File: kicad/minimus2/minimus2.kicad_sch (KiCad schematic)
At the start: 35 parts, among them J1 PROG_SER, J4 Conn_01x01, J5 Conn_01x01, J6 Conn_01x01, J7 Conn_01x01, Q1 DMN3051L, Q2 AO3401A, Q3 SFH309, Q4 SFH309, Q5 SFH309, Q6 SFH309, Q7 DMN3051L, Q8 DMN3051L, Q9 DMN3051L, SW1 USER_A, SW2 RESET, U1 DRV8835, U2 LSM6DSRTR, U4 AS5047D, U5 AS5047D, U6 STM32U575CITx

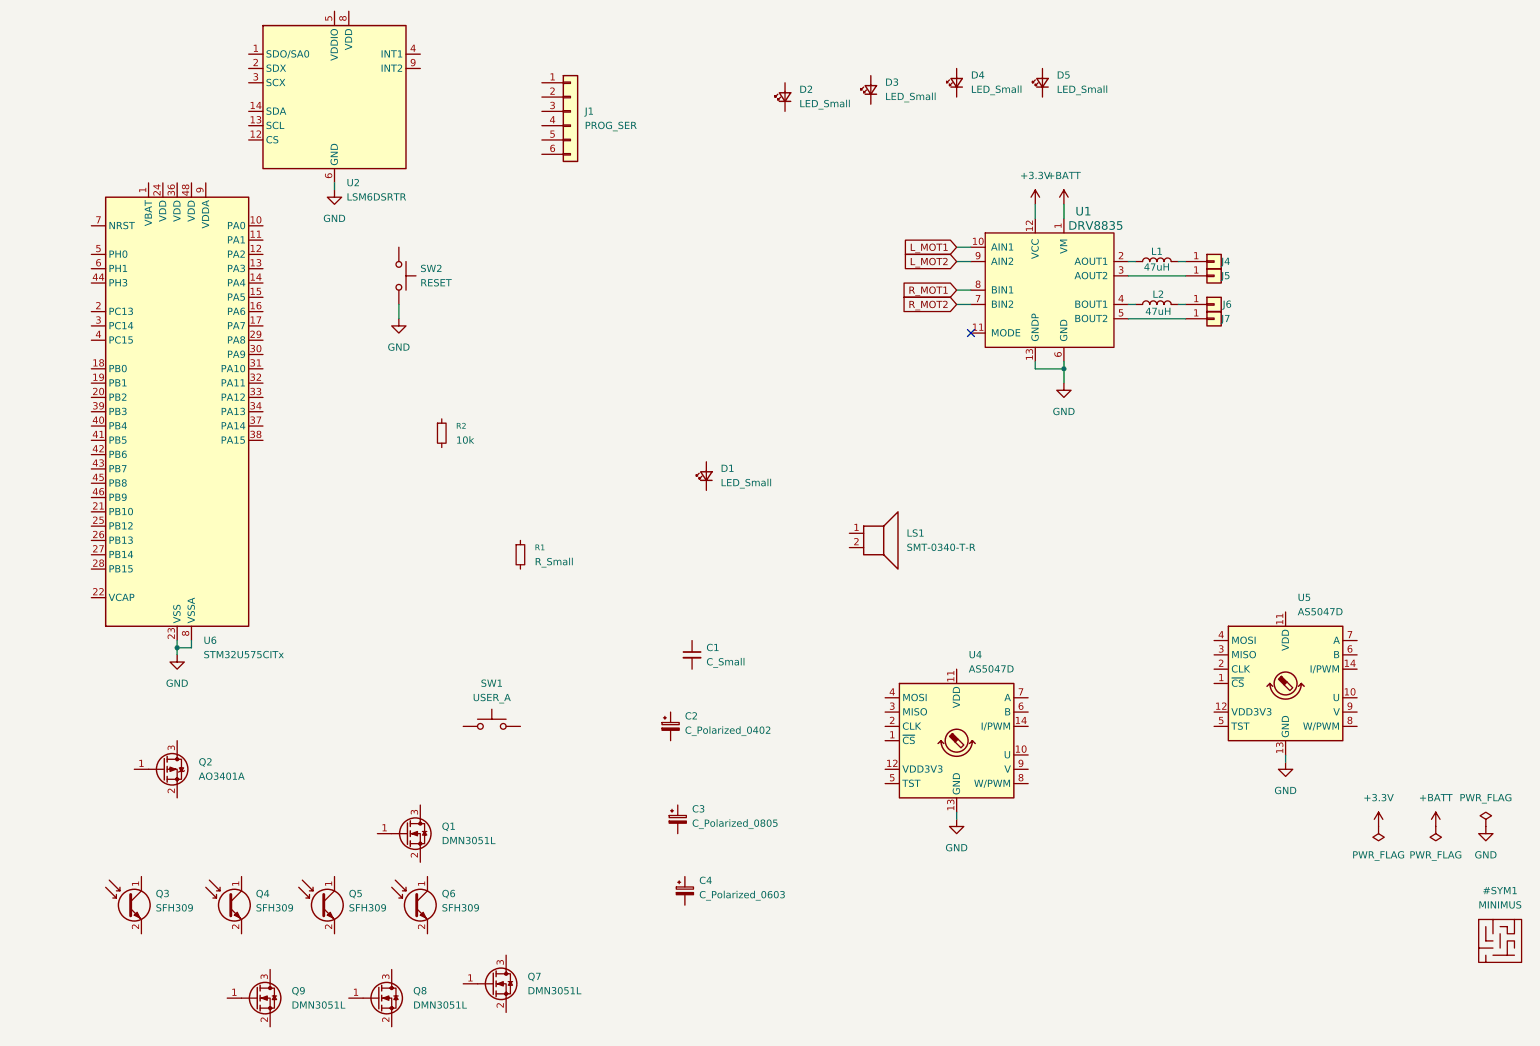
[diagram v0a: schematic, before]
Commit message: Rough place most parts
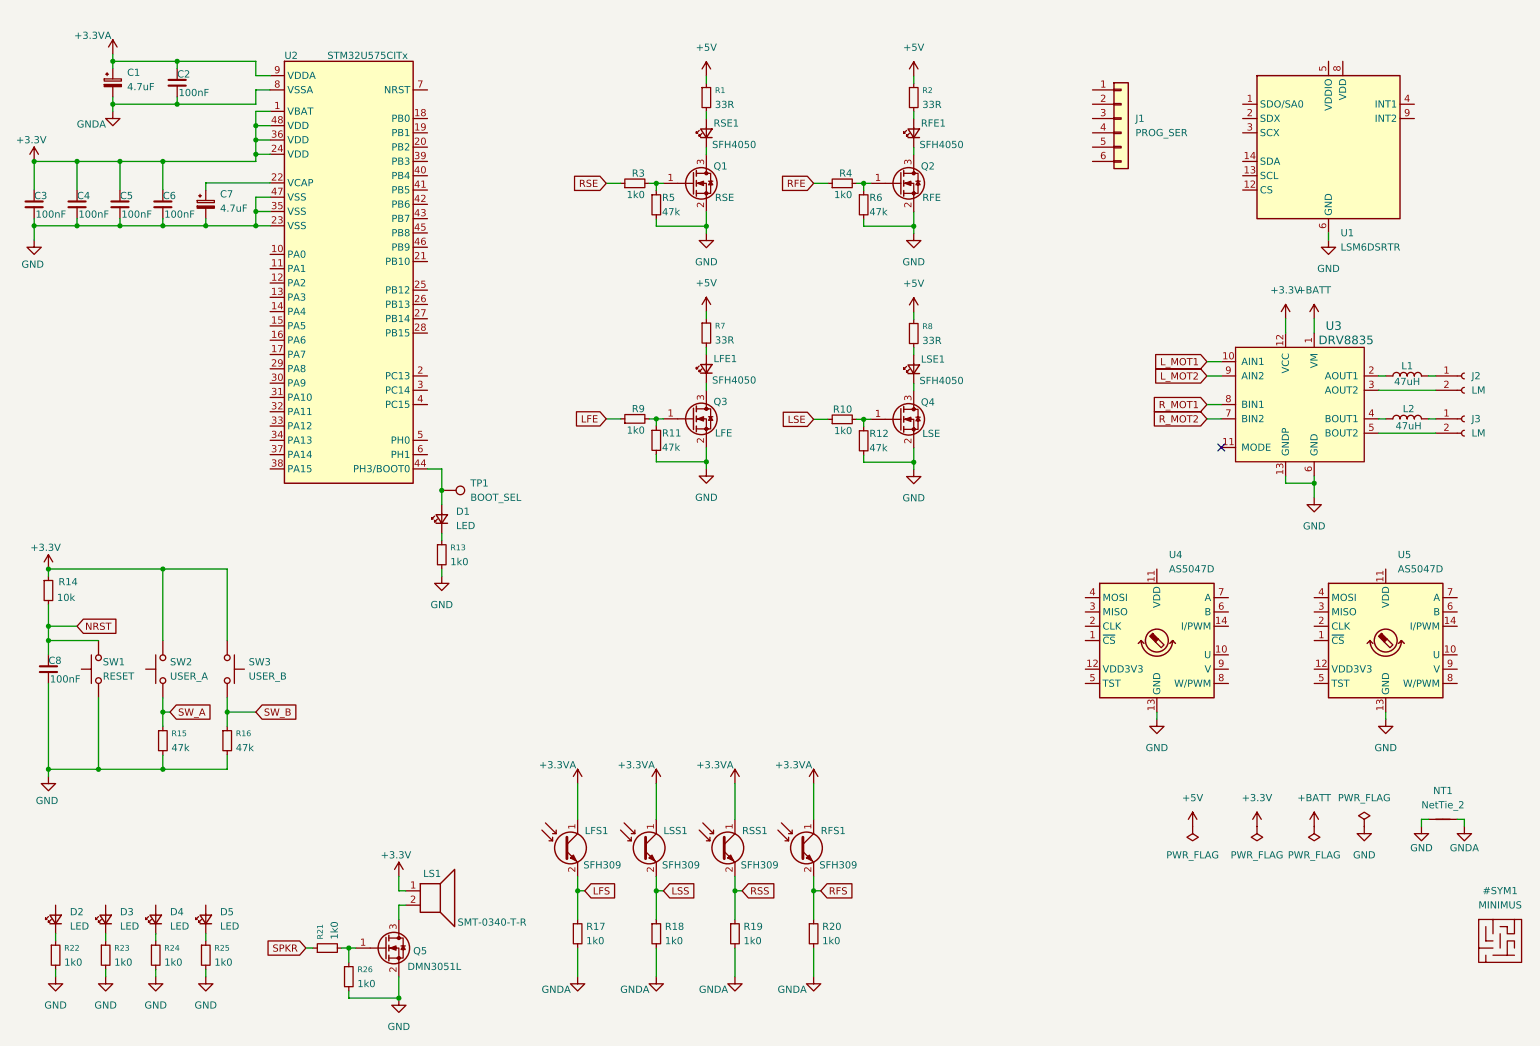
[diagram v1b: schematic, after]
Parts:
- removed C1: C_Small, Capacitor_SMD:C_0402_1005Metric, symbol Device:C_Small
- removed C2: C_Polarized_0402, Capacitor_SMD:C_0402_1005Metric, symbol Device:C_Polarized_Small
- removed C3: C_Polarized_0805, Capacitor_SMD:C_0805_2012Metric, symbol Device:C_Polarized_Small
- removed C4: C_Polarized_0603, Capacitor_SMD:C_0603_1608Metric, symbol Device:C_Polarized_Small
- removed J4, J6: Conn_01x01, minimus:Motor Red, symbol Connector_Generic:Conn_01x01
- removed J5, J7: Conn_01x01, minimus:Motor Blk, symbol Connector_Generic:Conn_01x01
- removed Q2: AO3401A, Package_TO_SOT_SMD:SOT-23, symbol Transistor_FET:AO3401A
- removed Q4, Q5, Q6: SFH309, LED_THT:LED_D3.0mm_Horizontal_O1.27mm_Z2.0mm_Clear, symbol Sensor_Optical:SFH309
- removed Q7, Q8, Q9: DMN3051L, Package_TO_SOT_SMD:SOT-23, symbol Transistor_FET:DMN3051L
- removed U6: STM32U575CITx, Package_QFP:LQFP-48_7x7mm_P0.5mm, symbol MCU_ST_STM32U5:STM32U575CITx
- added C1, C7: 4.7uF, Capacitor_SMD:C_0805_2012Metric, symbol Device:C_Polarized_Small
- added C2, C3, C4, C5, C6, C8: 100nF, Capacitor_SMD:C_0402_1005Metric, symbol minimus:C_Small
- added D5: LED, LED_SMD:LED_0402_1005Metric, symbol Device:LED_Small
- added J2, J3: LM, Connector_PinHeader_2.00mm:PinHeader_1x02_P2.00mm_Vertical, symbol Connector:Conn_01x02_Socket
- added LFE1, LSE1, RSE1: SFH4050, LED_THT:LED_D3.0mm_Horizontal_O1.27mm_Z2.0mm_IRBlack, symbol Device:LED_Small
- added LSS1, RFS1, RSS1: SFH309, LED_THT:LED_D3.0mm_Horizontal_O1.27mm_Z2.0mm_Clear, symbol Sensor_Optical:SFH309
- added NT1: NetTie_2, NetTie:NetTie-2_SMD_Pad0.5mm, symbol Device:NetTie_2
- added Q1: RSE, Package_TO_SOT_SMD:SOT-23, symbol Transistor_FET:DMN3051L
- added Q3: LFE, Package_TO_SOT_SMD:SOT-23, symbol Transistor_FET:DMN3051L
- added Q4: LSE, Package_TO_SOT_SMD:SOT-23, symbol Transistor_FET:DMN3051L
- added Q5: DMN3051L, Package_TO_SOT_SMD:SOT-23, symbol Transistor_FET:DMN3051L
- added R10, R13, R17, R18, R19, R20, R21, R22, R23, R24, R25, R26, R3, R4, R9: 1k0, Resistor_SMD:R_0402_1005Metric, symbol Device:R_Small
- added R11, R12, R15, R16, R5, R6: 47k, Resistor_SMD:R_0402_1005Metric, symbol Device:R_Small
- added R14: 10k, Resistor_SMD:R_0402_1005Metric, symbol Device:R_Small
- added R7, R8: 33R, Resistor_SMD:R_0402_1005Metric, symbol Device:R_Small
- added SW1: RESET, Button_Switch_SMD:SW_Push_1P1T_NO_CK_KMR2, symbol minimus:SW_Push
- added TP1: BOOT_SEL, TestPoint:TestPoint_Pad_D1.0mm, symbol Connector:TestPoint
- added U2: STM32U575CITx, Package_QFP:LQFP-48_7x7mm_P0.5mm, symbol minimus:STM32U575CITx-FUNC
- D1: value LED_Small -> LED
- D2, D3, D4: value LED_Small -> LED; footprint LED_THT:LED_D3.0mm_Horizontal_O1.27mm_Z2.0mm_IRBlack -> LED_SMD:LED_0402_1005Metric
- J1: footprint Connector_JST:JST_SH_BM06B-SRSS-TB_1x06-1MP_P1.00mm_Vertical -> Connector_PinHeader_1.27mm:PinHeader_2x03_P1.27mm_Vertical
- Q2: renamed from Q1; value DMN3051L -> RFE
- R1: value R_Small -> 33R
- R2: value 10k -> 33R; LCSC C25744 -> (none)
- RFE1: renamed from D5; value LED_Small -> SFH4050
- SW3: renamed from SW2; value RESET -> USER_B
- renumbered Q3 to LFS1, SW1 to SW2, U2 to U1, U1 to U3
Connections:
- net +3.3V: now also LS1.1, SW2.2, SW3.1, C3.1, C4.1, C5.1, C6.1, R14.1, U2.1 (VBAT), U2.24 (VDD), U2.36 (VDD), U2.48 (VDD)
- net GND: now also Q2.2 (S), C3.2, C4.2, C5.2, C6.2, C7.2, C8.2, NT1.1, Q1.2 (S), Q3.2 (S), Q4.2 (S), Q5.2 (S), R11.2, R12.2, R13.2, R15.2, R16.2, R22.2, R23.2, R24.2, R25.2, R26.2, R5.2, R6.2, SW1.1, U2.23 (VSS), U2.35 (VSS), U2.47 (VSS); no longer SW3.2
- net at L1.2: now also J2.1 (Pin_1)
- net SW_A: now reaches SW2.1
- net SW_A: now also R15.1
- net at U3.3 (AOUT2): now also J2.2 (Pin_2)
- net at U3.5 (BOUT2): now also J3.2 (Pin_2)
- net +3.3VA: now reaches LFS1.1 (C)
- net +3.3VA: now also C1.1, C2.1, LSS1.1 (C), RFS1.1 (C), RSS1.1 (C), U2.9 (VDDA)
- net LFS: now reaches LFS1.2 (E)
- net LFS: now also R17.1
- net +5V: now reaches R2.1
- net +5V: now also R1.1, R7.1, R8.1
- net at R2.2: now also RFE1.2 (A)
- net at R1.2: now also RSE1.2 (A)
- net at D1.1 (K): now also R13.1
- net at D1.2 (A): now also TP1.1, U2.44 (PH3/BOOT0)
- net at Q2.1 (G): now also R4.2, R6.1
- net at Q2.3 (D): now also RFE1.1 (K)
- net at L2.2: now also J3.1 (Pin_1)
- net at LS1.2: now also Q5.3 (D)
- net at D3.1 (K): now also R23.1
- net at D4.1 (K): now also R24.1
- net at D2.1 (K): now also R22.1
- new net: LSE1.1 (K), Q4.3 (D)
- new net: LSE1.2 (A), R8.2
- new net: Q3.1 (G), R11.1, R9.2
- new net: LFE1.1 (K), Q3.3 (D)
- new net: C7.1, U2.22 (VCAP)
- new net: Q1.1 (G), R3.2, R5.1
- new net: Q1.3 (D), RSE1.1 (K)
- new net: Q5.1 (G), R21.2, R26.1
- new net: Q4.1 (G), R10.2, R12.1
- new net: D5.1 (K), R25.1
- new net: LFE1.2 (A), R7.2
- new net GNDA: C1.2, C2.2, NT1.2, R17.2, R18.2, R19.2, R20.2, U2.8 (VSSA)
- new net LFE: R9.1
- new net LSE: R10.1
- new net LSS: LSS1.2 (E), R18.1
- new net NRST: C8.1, R14.2, SW1.2
- new net RFE: R4.1
- new net RFS: R20.1, RFS1.2 (E)
- new net RSE: R3.1
- new net RSS: R19.1, RSS1.2 (E)
- new net SPKR: R21.1
- new net SW_B: R16.1, SW3.2
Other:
- moved on the sheet: J1, L1, L2, LFS1, LS1, Q2, RFE1, SW2, SW3, U1, U3, U4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
